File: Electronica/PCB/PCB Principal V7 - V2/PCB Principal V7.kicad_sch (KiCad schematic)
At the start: 17 parts, among them J1 Conexion Sensores, J2 Power Monster, J3 On/Off General, J6 Power Input 1, SW1 On/Off Motores, SW2 SW_DIP_x05, SW3 SW_Push, U2 CD74HC4067M

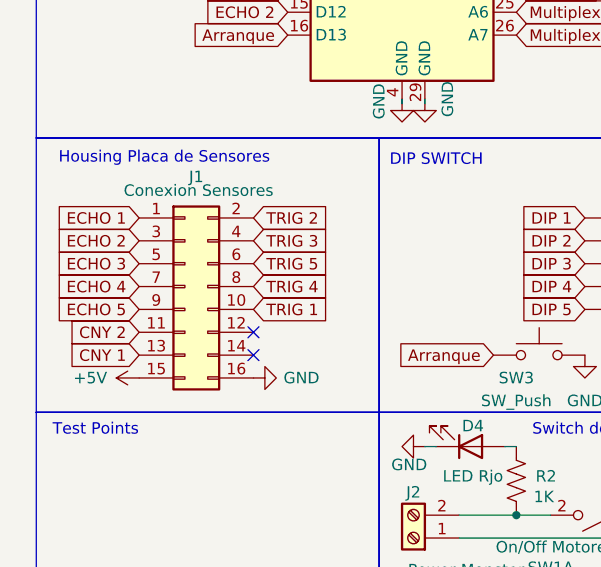
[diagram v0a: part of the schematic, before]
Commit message: Sensores V3
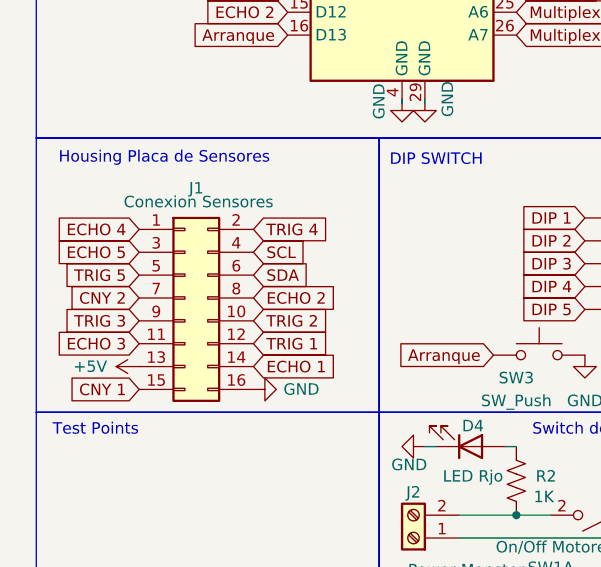
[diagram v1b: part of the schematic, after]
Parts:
- J1: footprint Connector_PinHeader_2.54mm:PinHeader_2x08_P2.54mm_Horizontal -> Connector_PinHeader_2.54mm:PinHeader_2x08_P2.54mm_Vertical
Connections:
- net +5V: now also J1.13 (Pin_13); no longer J1.15 (Pin_15)
- net CNY 1: now also J1.15 (Pin_15); no longer J1.13 (Pin_13)
- net CNY 2: now also J1.7 (Pin_7); no longer J1.11 (Pin_11)
- net ECHO 1: now also J1.14 (Pin_14); no longer J1.1 (Pin_1)
- net ECHO 2: now also J1.8 (Pin_8); no longer J1.3 (Pin_3)
- net ECHO 3: now also J1.11 (Pin_11); no longer J1.5 (Pin_5)
- net ECHO 4: now also J1.1 (Pin_1); no longer J1.7 (Pin_7)
- net ECHO 5: now also J1.3 (Pin_3); no longer J1.9 (Pin_9)
- net TRIG 1: now also J1.12 (Pin_12); no longer J1.10 (Pin_10)
- net TRIG 2: now also J1.10 (Pin_10); no longer J1.2 (Pin_2)
- net TRIG 3: now also J1.9 (Pin_9); no longer J1.4 (Pin_4)
- net TRIG 4: now also J1.2 (Pin_2); no longer J1.8 (Pin_8)
- net TRIG 5: now also J1.5 (Pin_5); no longer J1.6 (Pin_6)
- new net SCL: J1.4 (Pin_4)
- new net SDA: J1.6 (Pin_6)
- no-connect marks 9 -> 7

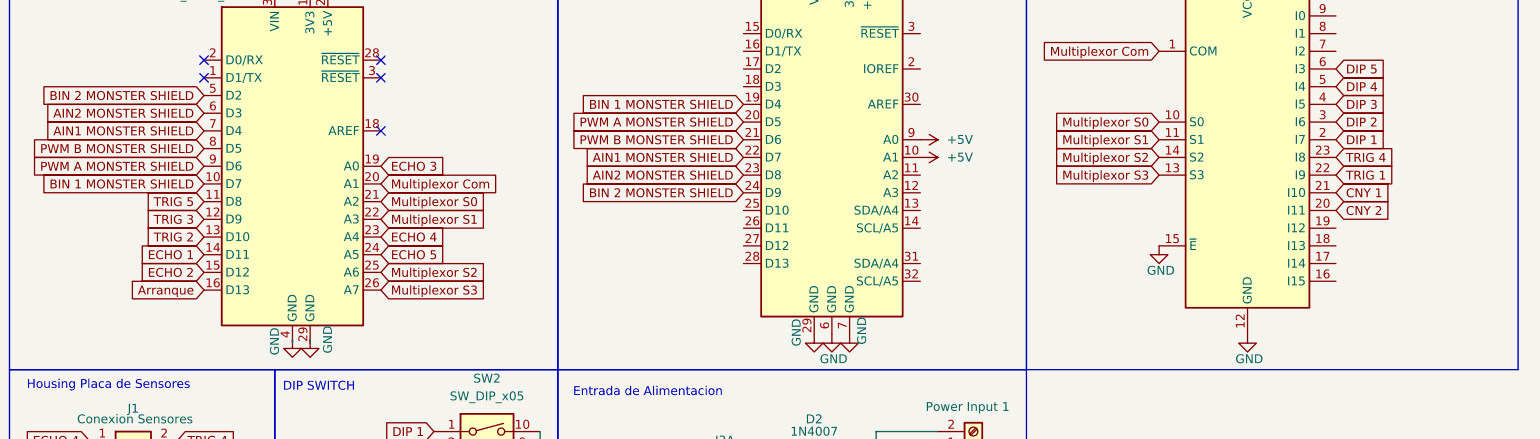
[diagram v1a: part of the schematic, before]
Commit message: Placa principal terminada
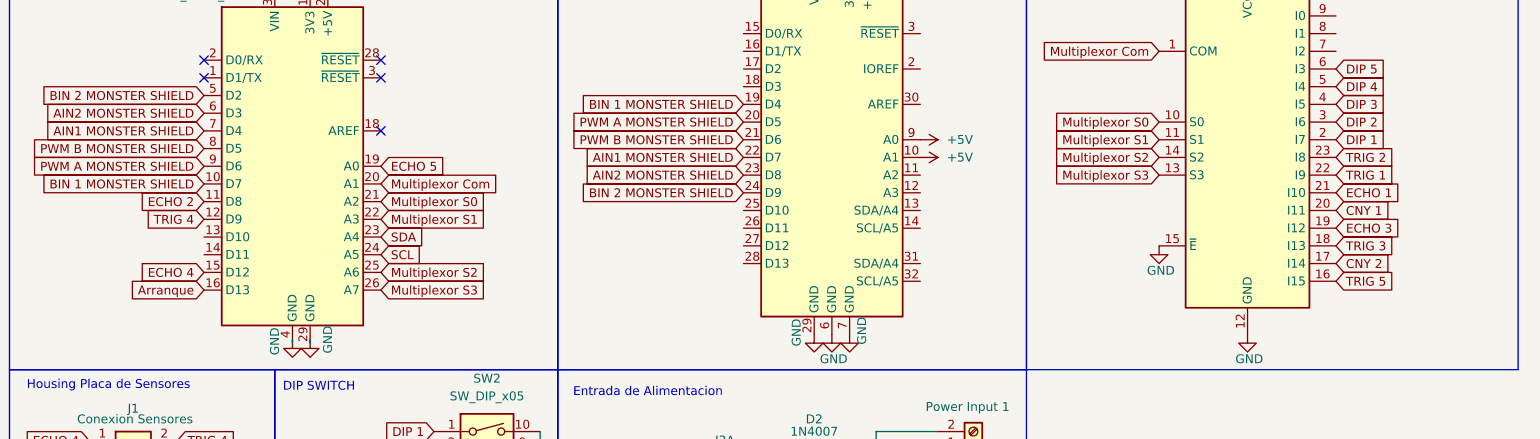
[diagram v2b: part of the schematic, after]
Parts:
- J1: footprint Connector_PinHeader_2.54mm:PinHeader_2x08_P2.54mm_Vertical -> Connector_PinHeader_2.54mm:PinHeader_2x08_P2.54mm_Horizontal
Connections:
- net CNY 1: now also U2.20 (I11); no longer U2.21 (I10)
- net CNY 2: now also U2.17 (I14); no longer U2.20 (I11)
- net ECHO 1: now also U2.21 (I10); no longer A1.14 (D11)
- net ECHO 2: now also A1.11 (D8); no longer A1.15 (D12)
- net ECHO 3: now also U2.19 (I12); no longer A1.19 (A0)
- net ECHO 4: now also A1.15 (D12); no longer A1.23 (A4)
- net ECHO 5: now also A1.19 (A0); no longer A1.24 (A5)
- net SCL: now also A1.24 (A5)
- net SDA: now also A1.23 (A4)
- net TRIG 2: now also U2.23 (I8); no longer A1.13 (D10)
- net TRIG 3: now also U2.18 (I13); no longer A1.12 (D9)
- net TRIG 4: now also A1.12 (D9); no longer U2.23 (I8)
- net TRIG 5: now also U2.16 (I15); no longer A1.11 (D8)

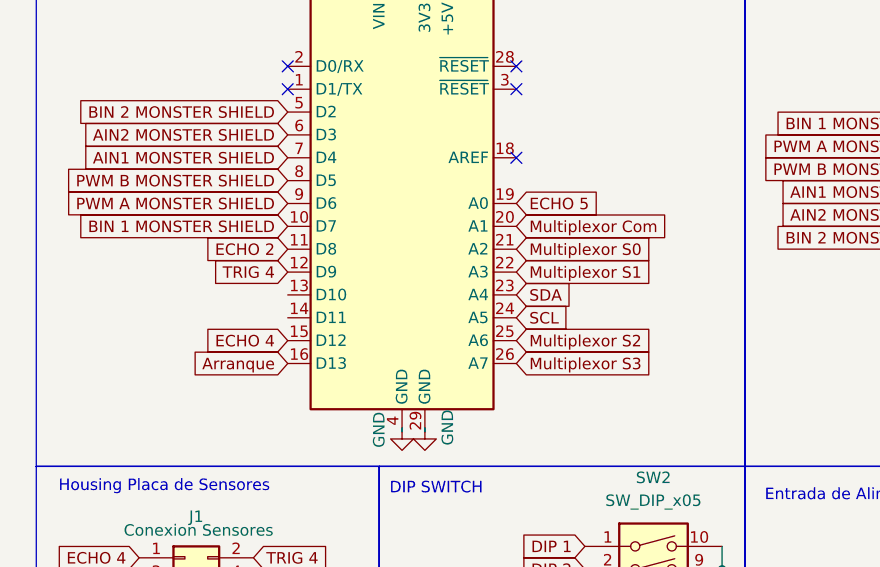
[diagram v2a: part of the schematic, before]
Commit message: teminada
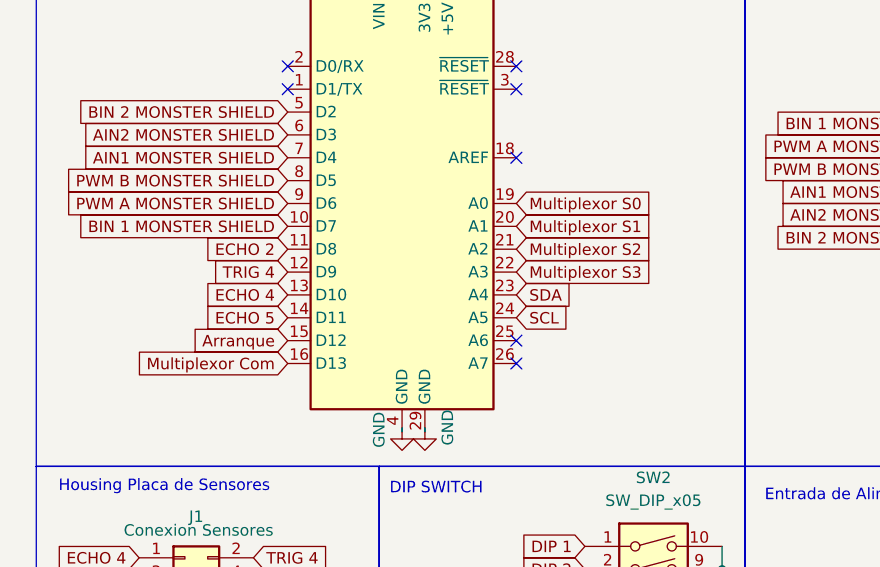
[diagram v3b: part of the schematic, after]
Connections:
- net Arranque: now also A1.15 (D12); no longer A1.16 (D13)
- net ECHO 4: now also A1.13 (D10); no longer A1.15 (D12)
- net ECHO 5: now also A1.14 (D11); no longer A1.19 (A0)
- net Multiplexor Com: now also A1.16 (D13); no longer A1.20 (A1)
- net Multiplexor S0: now also A1.19 (A0); no longer A1.21 (A2)
- net Multiplexor S1: now also A1.20 (A1); no longer A1.22 (A3)
- net Multiplexor S2: now also A1.21 (A2); no longer A1.25 (A6)
- net Multiplexor S3: now also A1.22 (A3); no longer A1.26 (A7)
- no-connect marks 7 -> 9
